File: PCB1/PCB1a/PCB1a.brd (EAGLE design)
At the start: 125.6 x 84.2 mm, 0 parts

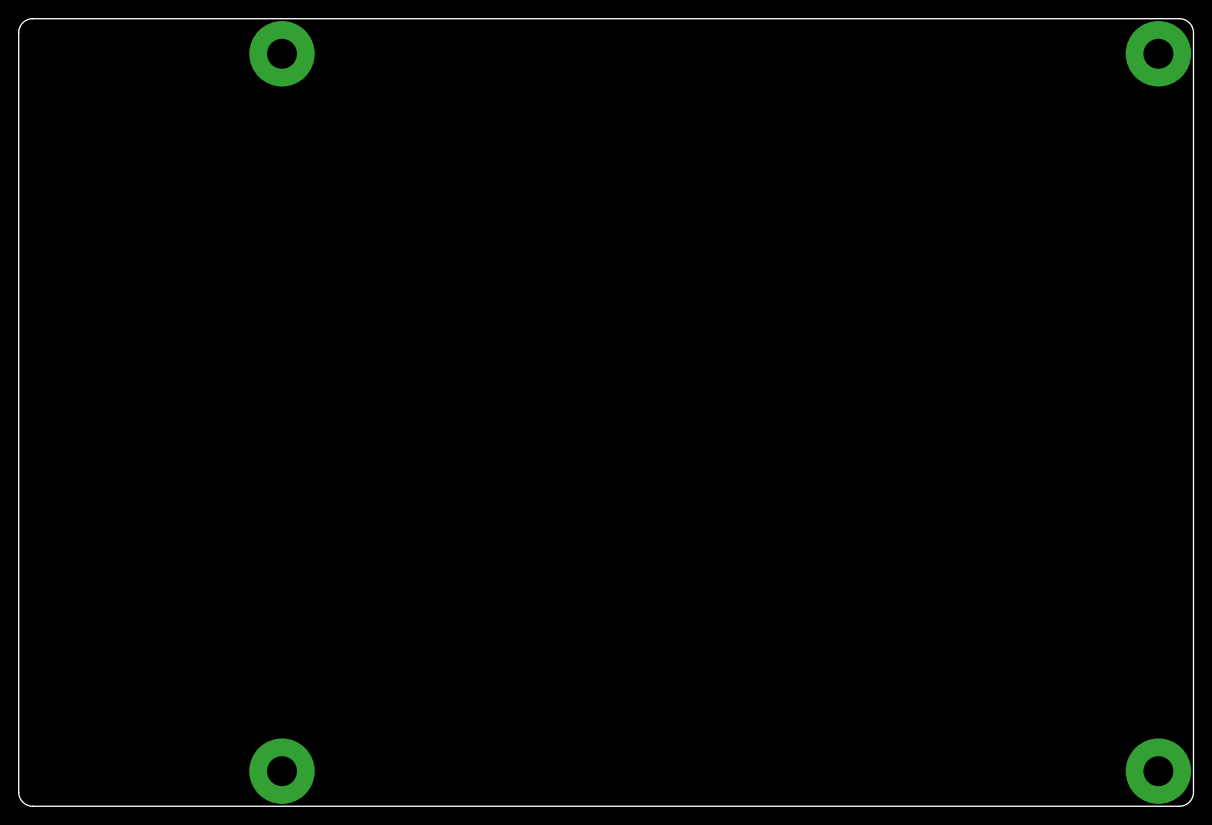
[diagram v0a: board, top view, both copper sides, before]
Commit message: .
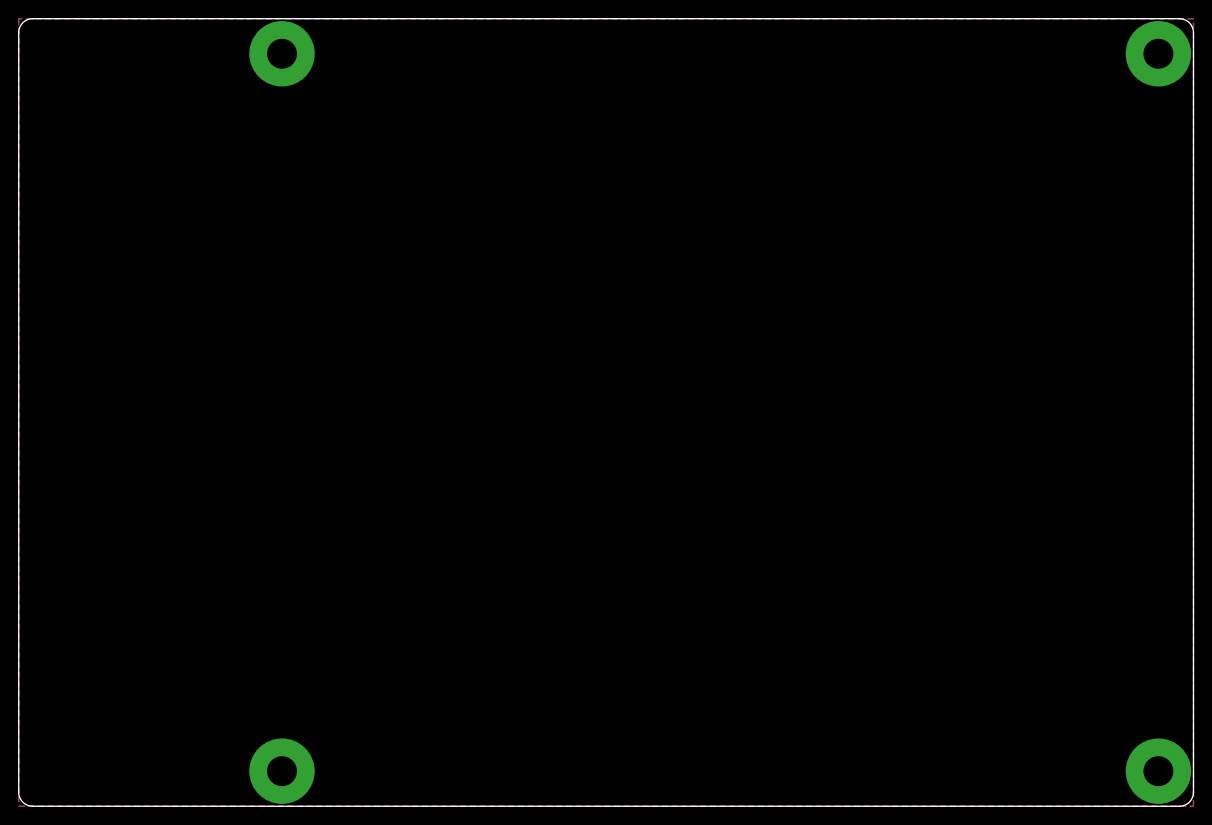
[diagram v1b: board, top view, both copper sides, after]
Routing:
- added copper zone on layer 1, net GND
- added copper zone on layer 16, net GND
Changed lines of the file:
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@@
 <setting verticaltext="up"/>
 </settings>
-<grid distance="3.75" unitdist="mm" unit="mm" style="lines" multiple="1" display="yes" altdistance="5" altunitdist="mil" altunit="mil"/>
+<grid distance="4" unitdist="mm" unit="mm" style="lines" multiple="1" display="yes" altdistance="5" altunitdist="mil" altunit="mil"/>
 <layers>
 <layer number="1" name="Top" color="4" fill="1" visible="yes" active="yes"/>
@@
 <layer number="51" name="tDocu" color="7" fill="1" visible="yes" active="yes"/>
 <layer number="52" name="bDocu" color="7" fill="1" visible="yes" active="yes"/>
+<layer number="91" name="Nets" color="2" fill="1" visible="no" active="no"/>
+<layer number="92" name="Busses" color="1" fill="1" visible="no" active="no"/>
+<layer number="93" name="Pins" color="2" fill="1" visible="no" active="no"/>
+<layer number="94" name="Symbols" color="4" fill="1" visible="no" active="no"/>
+<layer number="95" name="Names" color="7" fill="1" visible="no" active="no"/>
+<layer number="96" name="Values" color="7" fill="1" visible="no" active="no"/>
+<layer number="97" name="Info" color="7" fill="1" visible="no" active="no"/>
+<layer number="98" name="Guide" color="6" fill="1" visible="no" active="no"/>
 </layers>
 <board>
@@
 <dimension x1="50.6" y1="42.1" x2="50.6" y2="-42.1" x3="60.6" y3="0" textsize="1.778" layer="47"/>
 <dimension x1="50.6" y1="-42.1" x2="-75" y2="-42.1" x3="-12.2" y3="-52.1" textsize="1.778" layer="47"/>
+<rectangle x1="42.85" y1="34.35" x2="50.6" y2="42.1" layer="41"/>
+<rectangle x1="42.85" y1="34.35" x2="50.6" y2="42.1" layer="42"/>
 </plain>
 <attributes>
@@
 </elements>
 <signals>
-<signal name="S$1">
+<signal name="MOUNT2">
 <via x="46.85" y="38.35" extent="1-16" drill="3.2" diameter="7" locked="yes"/>
 <via x="46.85" y="-38.35" extent="1-16" drill="3.2" diameter="7" locked="yes"/>
@@
 <wire x1="-46.85" y1="38.35" x2="-46.85" y2="-38.35" width="0" layer="19" extent="1-1"/>
 </signal>
+<signal name="GND">
+<polygon width="0.1524" layer="1">
+<vertex x="50.6" y="-42.1"/>
+<vertex x="50.6" y="42.1"/>
+<vertex x="-75" y="42.1"/>
+<vertex x="-75" y="-42.1"/>
+</polygon>
+<polygon width="0.1524" layer="16">
+<vertex x="50.6" y="-42.1"/>
+<vertex x="50.6" y="42.1"/>
+<vertex x="-75" y="42.1"/>
+<vertex x="-75" y="-42.1"/>
+</polygon>
+</signal>
 </signals>
